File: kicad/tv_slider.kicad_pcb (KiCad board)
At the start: 2 copper layers, 131.5 x 79.5 mm, 96 parts, among them J1 MC 1,5/2-G-3.81, J2 MC 1,5/6-G-3.81, J3 MC 1,5/4-G-3.81, J4 MC 1,5/3-G-3.81, J5 MC 1,5/3-G-3.81, J6 MC 1,5/3-G-3.81, J7 MC 1,5/3-G-3.81, J8 Conn_01x04, Q1 CSD19537Q3, Q2 BSS138, U1 TPS26632RGE, U2 LMR33610ADDAR, U3 LMR33610ADDAR, U4 ESP32-C6-DEVKITC-1-N8, U5 DRV8452DDWR, U6 ISL3280ExHZ, U7 LS7184N-S, U8 ISL3280ExHZ

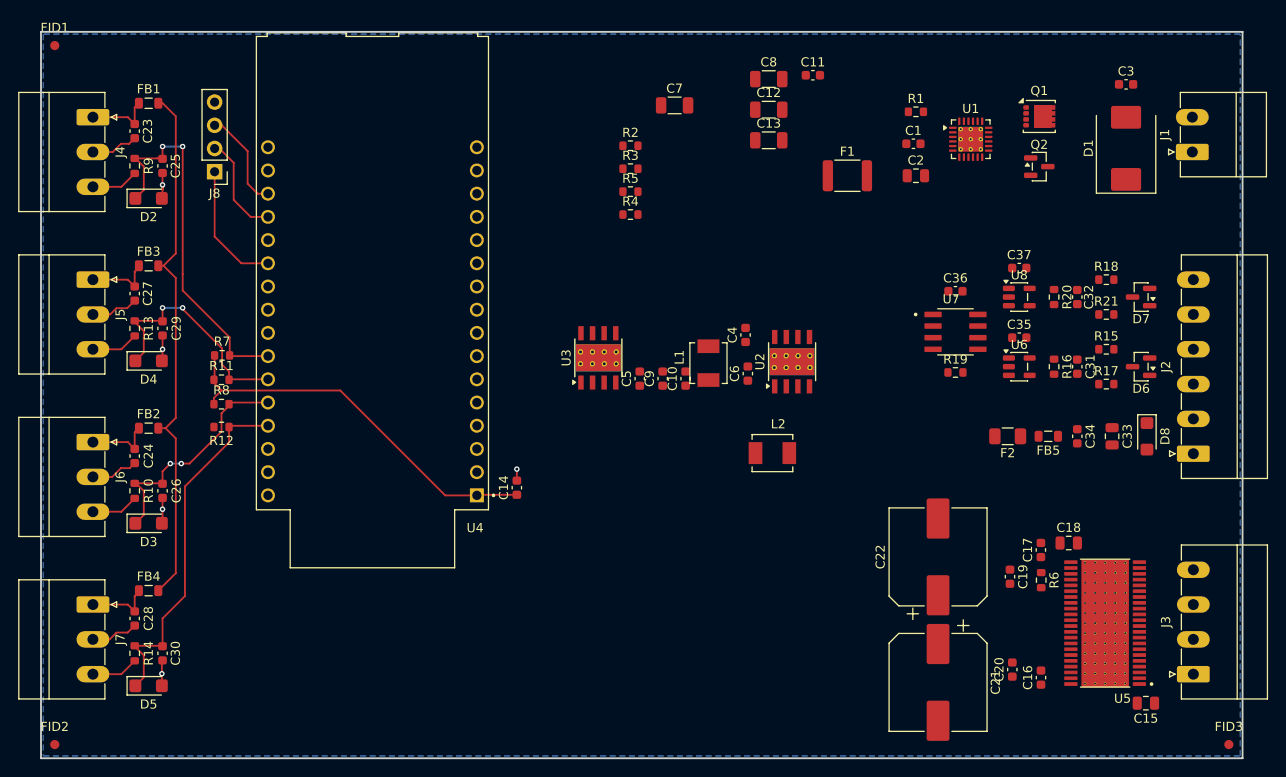
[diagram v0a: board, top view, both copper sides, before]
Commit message: Completed the PCB design. Ready for final review.
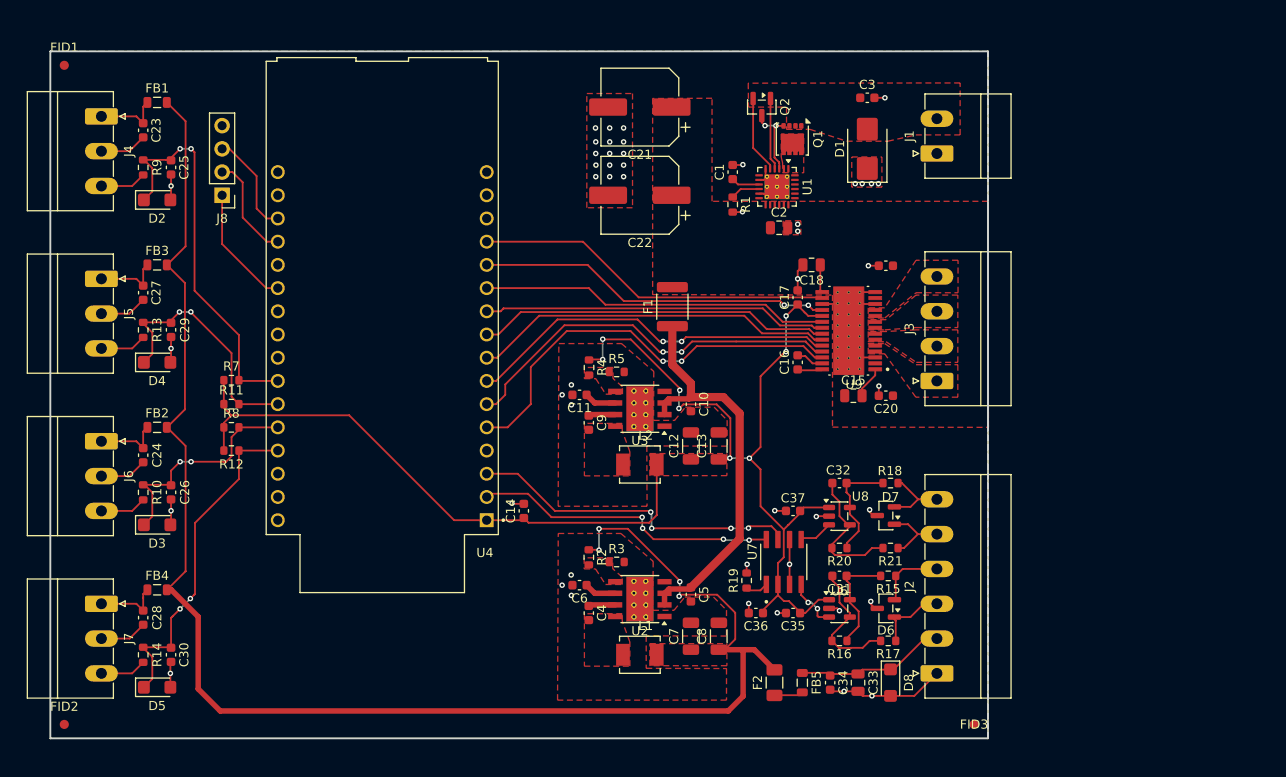
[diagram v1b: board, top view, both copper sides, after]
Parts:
- removed R6: 100k, Resistor_SMD:R_0603_1608Metric
- removed U5: DRV8452DDWR, local_library:IC_DRV8452DDWR
- added U9: DRV8452SPWPR, local_library:IC_DRV8452SPWPR, F.Cu at (168.1, 87.0)
- C21, C22: value 150u -> 100u; footprint Capacitor_SMD:CP_Elec_10x12.5 -> Capacitor_SMD:CP_Elec_8x11.9
- D1: value 1.5SMC33CA -> SMBJ33CA; footprint Diode_SMD:D_SMC -> Diode_SMD:D_SMB
- moved C21 70.9 mm to (145.3, 62.5), turned to 180 degrees
- moved C8 61.2 mm to (153.9, 120.4), turned to 90 degrees
- moved C7 58.1 mm to (150.9, 120.4), turned to 90 degrees
- moved C22 51.3 mm to (145.3, 72.1), turned to 180 degrees
- moved C15 46.4 mm to (168.7, 94.1), turned to 0 degrees
- moved R2 45.3 mm to (139.7, 111.8), turned to -90 degrees
- moved C16 43.6 mm to (162.6, 90.4)
- moved C11 43.3 mm to (138.7, 94.0), turned to 180 degrees
- moved R3 43.1 mm to (142.7, 112.3)
- moved J3 42.6 mm to (177.8, 92.5)
- moved C18 41.5 mm to (164.1, 79.8), turned to 180 degrees
- moved C36 41.4 mm to (158.0, 117.9), turned to 180 degrees
- moved C35 39.0 mm to (162.1, 117.9), turned to 180 degrees
- moved D8 38.9 mm to (172.7, 125.5)
- moved C33 38.7 mm to (169.2, 125.5)
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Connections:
- C12 pad 1: +3.3V -> +3V3
- C13 pad 1: +3.3V -> +3V3
- J3 pad 1: /Motor drive/B- -> /Motor drive/A+
- J3 pad 2: /Motor drive/B+ -> /Motor drive/A-
- J3 pad 3: /Motor drive/A- -> /Motor drive/B-
- J3 pad 4: /Motor drive/A+ -> /Motor drive/B+
- L2 pad 2: +3.3V -> +3V3
- R4 pad 1: +3.3V -> +3V3
- U4 pad J1_10: unconnected-(U4-GPIO10-PadJ1_10) -> /MCU/MOSI
- U4 pad J1_11: unconnected-(U4-GPIO11-PadJ1_11) -> /MCU/MISO
- U4 pad J1_12: unconnected-(U4-GPIO2-PadJ1_12) -> /MCU/~{CS}
- U4 pad J1_13: unconnected-(U4-GPIO3-PadJ1_13) -> /MCU/~{FAULT}
- U4 pad J1_2: unconnected-(U4-CHIP_PU-PadJ1_2) -> /MCU/COUNT
- U4 pad J1_3: unconnected-(U4-GPIO4-PadJ1_3) -> /MCU/UP/~{DOWN}
- U4 pad J1_5: unconnected-(U4-GPIO6-PadJ1_5) -> /MCU/~{SLEEP}
- U4 pad J1_6: unconnected-(U4-GPIO7-PadJ1_6) -> /MCU/ENABLE
- U4 pad J1_7: unconnected-(U4-GPIO0-PadJ1_7) -> /MCU/DIR
- U4 pad J1_8: unconnected-(U4-GPIO1-PadJ1_8) -> /MCU/STEP
- U4 pad J1_9: unconnected-(U4-GPIO8-PadJ1_9) -> /MCU/SCLK
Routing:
- net +5V: track 58.6 -> 173.1 mm, vias 0 -> 4
- net +3V3: track 43.2 -> 152.8 mm, vias 0 -> 8
- net /MCU/~{SLEEP}: track 0.00 -> 46.0 mm, vias 0 -> 2
- net GND: track 34.4 -> 80.0 mm, vias 5 -> 49
- net Net-(U2-EN): track 0.00 -> 44.8 mm
- net /MCU/ENABLE: track 0.00 -> 43.1 mm, vias 0 -> 2
- net /MCU/DIR: track 0.00 -> 41.1 mm, vias 0 -> 2
- net /MCU/STEP: track 0.00 -> 39.7 mm
- net /MCU/~{FAULT}: track 0.00 -> 39.3 mm
- net /MCU/~{CS}: track 0.00 -> 38.8 mm, vias 0 -> 2
- net /MCU/SCLK: track 0.00 -> 38.7 mm
- net /MCU/MISO: track 0.00 -> 38.3 mm
- net /MCU/MOSI: track 0.00 -> 37.7 mm
- net /MCU/UP/~{DOWN}: track 0.00 -> 36.5 mm, vias 0 -> 4
- net /MCU/COUNT: track 0.00 -> 33.6 mm, vias 0 -> 4
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- added copper zone on F.Cu, net +3V3
- added copper zone on F.Cu, net +5V
- added copper zone on F.Cu, net /Motor drive/A+
- added copper zone on F.Cu, net /Motor drive/A-
- added copper zone on F.Cu, net /Motor drive/B+
- added copper zone on F.Cu, net /Motor drive/B-
- added copper zone on F.Cu, net /Power supply/Vin
- added copper zone on F.Cu, net GND
- added copper zone on F.Cu, net Net-(Q1-D)
- added copper zone on F.Cu, net Net-(U2-FB)
- added copper zone on F.Cu, net Net-(U2-SW)
- added copper zone on F.Cu, net Net-(U3-FB)
- added copper zone on F.Cu, net Net-(U3-SW)
- added copper zone on F.Cu, net Vdrive
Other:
- board size 131.5 x 79.5 mm -> 102.6 x 75.2 mm
- board text added: "TV-Slider - 1.0 Copyright (c) 2025"
